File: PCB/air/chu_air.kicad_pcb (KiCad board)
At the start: 2 copper layers, 210 x 10 mm, 24 parts, among them J1 Conn_01x06_Socket, Q1 Q_Photo_NPN, Q2 Q_Photo_NPN, Q3 Q_Photo_NPN, Q4 Q_Photo_NPN, Q5 Q_Photo_NPN, Q6 Q_Photo_NPN

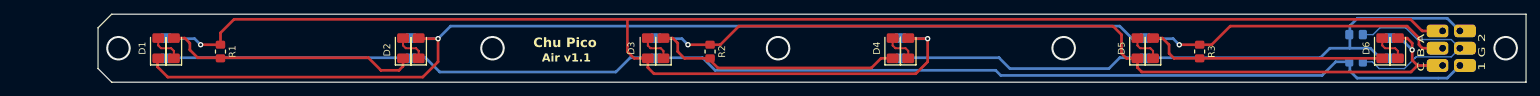
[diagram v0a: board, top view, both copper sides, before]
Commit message: Another attempt of chu air
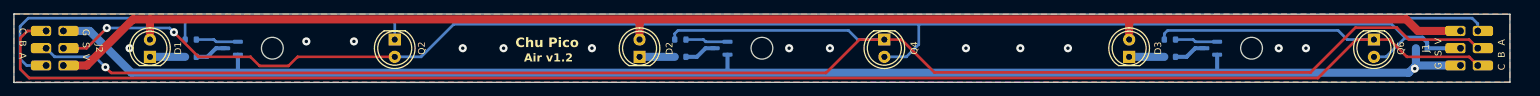
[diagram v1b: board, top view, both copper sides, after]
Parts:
- removed D10, D11, D12, D4, D5, D6, D7, D8, D9: IR26-21C_L110_TR8, LED_SMD:LED_1206_3216Metric_Pad1.42x1.75mm_HandSolder
- added J2: Conn_01x06_Socket, chu_air:6P_Air_Conn, F.Cu at (48.6, 97.5)
- added R6: 1R, Resistor_SMD:R_0603_1608Metric, B.Cu at (212.6, 98.8)
- added R7: 10K, Resistor_SMD:R_0603_1608Metric, B.Cu at (249.6, 97.5)
- D1, D2, D3: footprint LED_SMD:LED_1206_3216Metric_Pad1.42x1.75mm_HandSolder -> LED_THT:LED_D5.0mm_IRGrey
- J1: moved to F.Cu
- Q1, Q3, Q5: value Q_Photo_NPN -> AO3400A; footprint LED_SMD:LED_1206_3216Metric_Pad1.42x1.75mm_HandSolder -> Package_TO_SOT_SMD:SOT-23
- Q2, Q4, Q6: footprint LED_SMD:LED_1206_3216Metric_Pad1.42x1.75mm_HandSolder -> LED_THT:LED_D5.0mm_IRBlack; moved to F.Cu
- R1, R3: value R -> 10R; footprint Resistor_SMD:R_0805_2012Metric_Pad1.20x1.40mm_HandSolder -> Resistor_SMD:R_0603_1608Metric; moved to B.Cu
- R2: value R -> 1R; footprint Resistor_SMD:R_0805_2012Metric_Pad1.20x1.40mm_HandSolder -> Resistor_SMD:R_0603_1608Metric; moved to B.Cu
- R4: value R -> 1R; footprint Resistor_SMD:R_0805_2012Metric_Pad1.20x1.40mm_HandSolder -> Resistor_SMD:R_0603_1608Metric
- R5: value R -> 10R; footprint Resistor_SMD:R_0805_2012Metric_Pad1.20x1.40mm_HandSolder -> Resistor_SMD:R_0603_1608Metric
- moved R4 99.4 mm to (140.6, 98.8), turned to 180 degrees
- moved R3 76.4 mm to (140.6, 96.2), turned to 0 degrees
- moved R2 76.4 mm to (68.6, 98.8), turned to 180 degrees
- moved D3 68.5 mm to (206.6, 98.8)
- moved D2 34.8 mm to (134.6, 98.8)
- moved R5 27.4 mm to (212.6, 96.2)
- moved Q1 9.63 mm to (74.6, 97.5), turned to 180 degrees
- moved Q3 9.63 mm to (146.6, 97.5), turned to 180 degrees
- moved Q5 9.63 mm to (218.6, 97.5), turned to 180 degrees
- moved R1 4.71 mm to (68.6, 96.2), turned to 0 degrees
- moved D1 3.74 mm to (62.6, 98.8)
- moved Q2 2.69 mm to (98.6, 96.2)
- moved Q4 2.69 mm to (170.6, 96.2)
- moved Q6 2.69 mm to (242.6, 96.2)
- moved J1 2.63 mm to (256.6, 97.5)
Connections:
- D1 pad 2: Net-(D1-A) -> +3.3V
- D2 pad 1: Net-(D1-A) -> Net-(D2-K)
- D2 pad 2: Net-(D2-A) -> +3.3V
- D3 pad 2: Net-(D3-A) -> +3.3V
- J1 pad 4: /AD2 -> +3.3V
- J1 pad 5: GND -> /SIG
- J1 pad 6: /AD1 -> GND
- Q1 pad 1: /A -> Net-(Q1-G)
- Q1 pad 2: /AD1 -> GND
- Q2 pad 1: /B -> /A
- Q2 pad 2: /AD1 -> /SIG
- Q3 pad 1: /C -> Net-(Q3-G)
- Q3 pad 2: /AD1 -> GND
- Q4 pad 1: /A -> /B
- Q4 pad 2: /AD2 -> /SIG
- Q5 pad 1: /B -> Net-(Q5-G)
- Q5 pad 2: /AD2 -> GND
- Q6 pad 2: /AD2 -> /SIG
- R1 pad 2: Net-(D1-A) -> Net-(Q1-G)
- R2 pad 1: /C -> Net-(Q1-D)
- R2 pad 2: Net-(D3-A) -> Net-(D1-K)
- R3 pad 2: Net-(D5-A) -> Net-(Q3-G)
- R4 pad 1: /AD1 -> Net-(Q3-D)
- R4 pad 2: GND -> Net-(D2-K)
- R5 pad 1: /AD2 -> /C
- R5 pad 2: GND -> Net-(Q5-G)
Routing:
- net /SIG: track 0.00 -> 228.1 mm, vias 0 -> 2
- net +3.3V: track 0.00 -> 217.0 mm
- net /AD1: track 196.5 -> 0.00 mm
- net GND: track 32.2 -> 219.0 mm, vias 0 -> 14
- net /C: track 132.8 -> 260.1 mm, vias 2 -> 0
- net /AD2: track 95.2 -> 0.00 mm
- net /B: track 206.9 -> 252.5 mm, vias 2 -> 1
- net Net-(D1-A): track 37.6 -> 0.00 mm
- net Net-(D3-A): track 36.8 -> 0.00 mm
- net Net-(D5-A): track 35.7 -> 0.00 mm
- net /A: track 253.4 -> 231.6 mm, vias 2 -> 0
- net Net-(Q1-G): track 0.00 -> 6.25 mm
- net Net-(Q5-G): track 0.00 -> 6.25 mm
- net Net-(Q3-G): track 0.00 -> 6.25 mm
- net Net-(D2-K): track 0.00 -> 5.18 mm
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- added copper zone on B.Cu, net GND
- added copper zone on F.Cu, net GND
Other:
- board size 210 x 10 mm -> 220 x 10.1 mm
- board text added: "Air v1.2"
- board text added: "C B A"
- board text added: "G S V"
- board text removed: "Air v1.1"
